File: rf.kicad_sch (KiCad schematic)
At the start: 59 parts, among them IC1 SX1255IWLTRT, J1 Antenna, U11 PE4312, U2 PE4312, U7 GRF5604, U9 SKY13330-397LF, Y1 32MHz

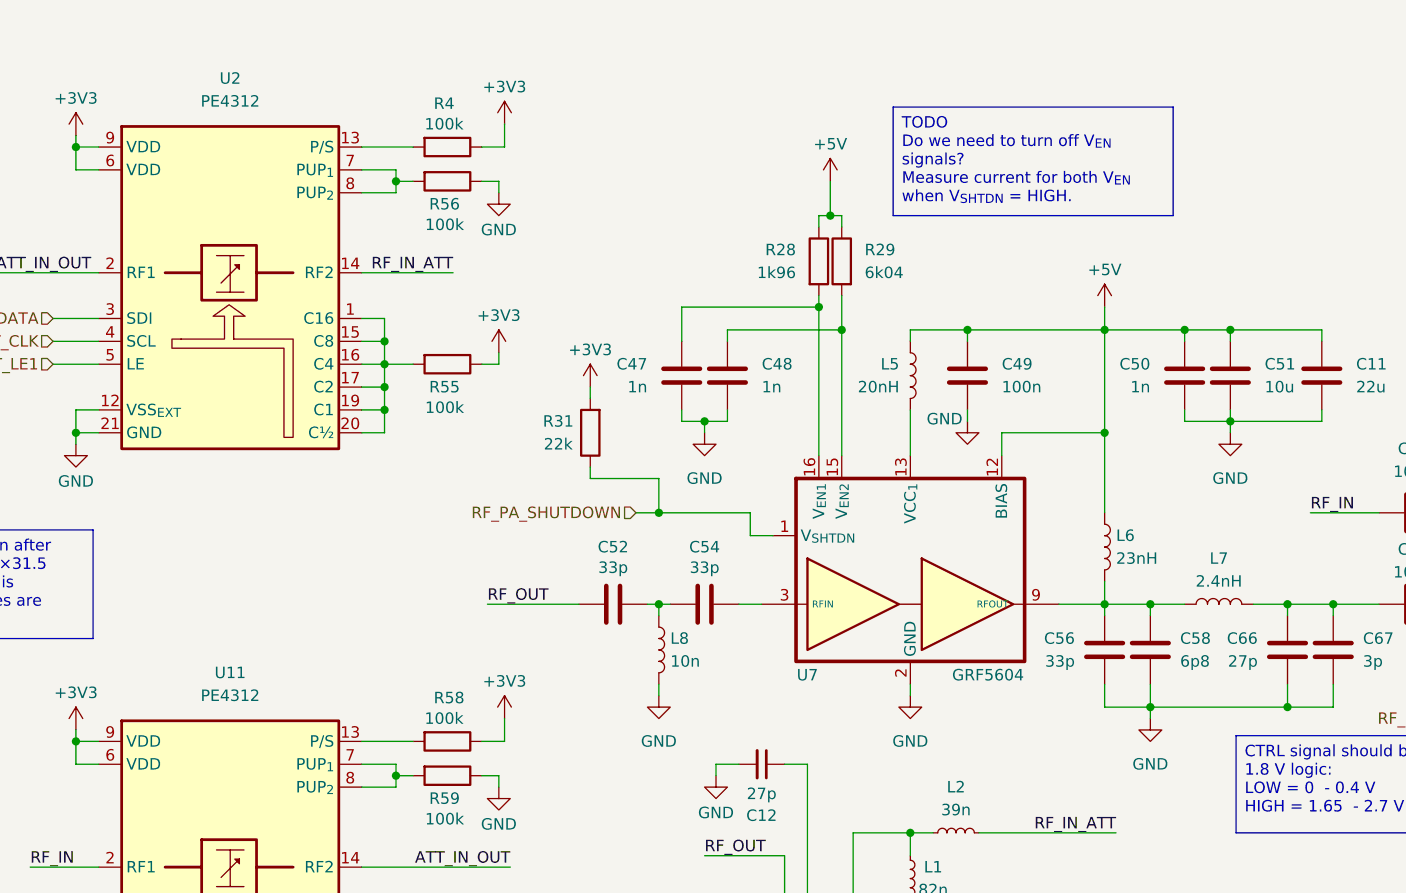
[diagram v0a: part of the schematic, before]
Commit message: Add `RF_PA_ENABLE` signal and MOSFETs to enable GRF5604
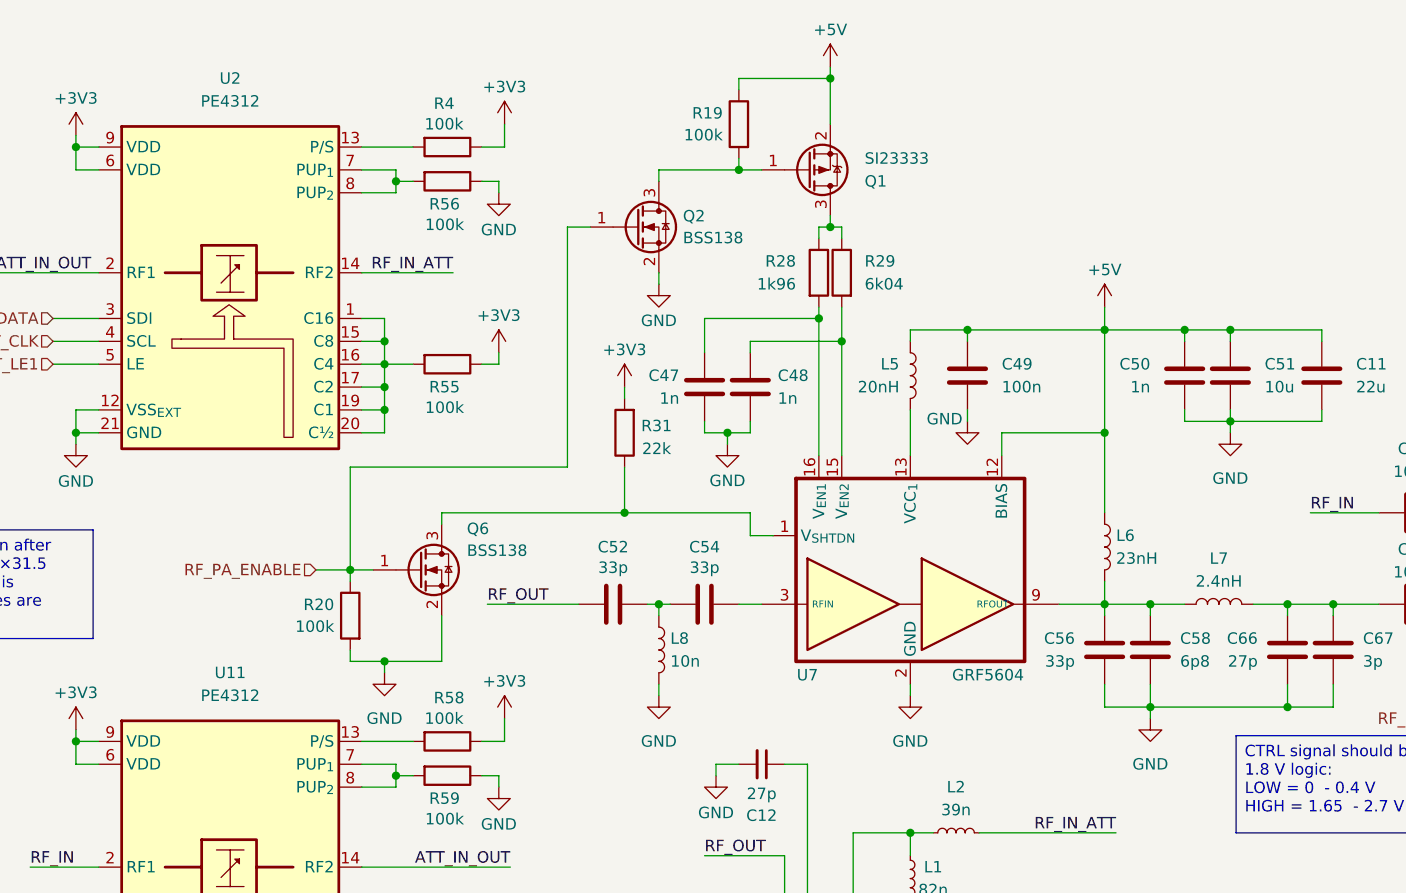
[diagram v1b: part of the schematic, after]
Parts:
- added Q1: SI23333, Package_TO_SOT_SMD:SOT-23, symbol Transistor_FET:Si2319CDS
- added Q2, Q6: BSS138, Package_TO_SOT_SMD:SOT-23, symbol Transistor_FET:BSS138
- added R19, R20: 100k, Resistor_SMD:R_0402_1005Metric, symbol Device:R
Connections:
- net +5V: now also Q1.2 (S), R19.1; no longer R28.1, R29.1
- net GND: now also Q2.2 (S), Q6.2 (S), R20.2
- net RF_PA_SHUTDOWN: no longer names the net of R31.1, U7.1 (V_{SHTDN})
- net RF_PA_SHUTDOWN: now also Q6.3 (D)
- new net: Q1.1 (G), Q2.3 (D), R19.2
- new net: Q1.3 (D), R28.1, R29.1
- new net RF_PA_ENABLE: Q2.1 (G), Q6.1 (G), R20.1
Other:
- moved on the sheet: C47, C48, R28, R29, R31

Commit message: Fix LCSC number of the GRF5604
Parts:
- U7: LCSC GRF5604 -> (none)
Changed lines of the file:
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@@
 		(on_board yes)
 		(dnp no)
-		(fields_autoplaced yes)
 		(property "Reference" "#PWR0146"
 			(at 82.55 91.44 0)
@@
 			)
 		)
-		(property "LCSC" "GRF5604"
+		(property "LCSC" ""
 			(at 147.32 77.47 0)
 			(effects

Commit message: Remove whitespaces in PN and MPN fields
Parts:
- C1, C2, C3, C4: PN 187-CL05B103KO5NNNC -> 187-CL05B103KO5NNNC
- C10, C13, C49, C5, C6, C7, C8, C9: PN 187-CL05B104KO5NNNC -> 187-CL05B104KO5NNNC
- C11: PN 187-CL31B226KPHNNNE -> 187-CL31B226KPHNNNE
- C12, C66: PN 603-CC402JRNPO9BN270 -> 603-CC402JRNPO9BN270
- C15, C47, C48, C50: PN 603-CC402JRNPO9BN102 -> 603-CC402JRNPO9BN102
- C51: PN 187-CL05A106MQ5NUNC -> 187-CL05A106MQ5NUNC
- IC1: PN 947-SX1255IWLTRT -> 947-SX1255IWLTRT
- Q2, Q6: PN 621-BSS138-7-F -> 621-BSS138-7-F
- U11, U2: PN 81-PE4312C-Z -> 81-PE4312C-Z
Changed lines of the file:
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@@
 			)
 		)
-		(property "PN" " 187-CL05B104KO5NNNC "
+		(property "PN" "187-CL05B104KO5NNNC"
 			(at 95.25 154.94 0)
 			(effects
@@
 			)
 		)
-		(property "PN" " 187-CL05B103KO5NNNC "
+		(property "PN" "187-CL05B103KO5NNNC"
 			(at 222.25 142.24 0)
 			(effects
@@
 			)
 		)
-		(property "PN" " 187-CL05B104KO5NNNC "
+		(property "PN" "187-CL05B104KO5NNNC"
 			(at 151.13 123.19 0)
 			(effects
@@
 			)
 		)
-		(property "PN" " 187-CL05A106MQ5NUNC "
+		(property "PN" "187-CL05A106MQ5NUNC"
 			(at 176.53 52.07 0)
 			(effects
@@
 			)
 		)
-		(property "PN" " 187-CL05B104KO5NNNC "
+		(property "PN" "187-CL05B104KO5NNNC"
 			(at 147.32 52.07 0)
 			(effects
@@
 			)
 		)
-		(property "PN" "81-PE4312C-Z "
+		(property "PN" "81-PE4312C-Z"
 			(at 50.8 92.71 0)
 			(effects
@@
 			)
 		)
-		(property "PN" " 187-CL05B104KO5NNNC "
+		(property "PN" "187-CL05B104KO5NNNC"
 			(at 271.78 142.24 0)
 			(effects
@@
 			)
 		)
-		(property "PN" " 187-CL05B104KO5NNNC "
+		(property "PN" "187-CL05B104KO5NNNC"
 			(at 77.47 154.94 0)
 			(effects
@@
 			)
 		)
-		(property "PN" " 187-CL05B104KO5NNNC "
+		(property "PN" "187-CL05B104KO5NNNC"
 			(at 260.35 142.24 0)
 			(effects
@@
 			)
 		)
-		(property "PN" " 603-CC402JRNPO9BN270 "
+		(property "PN" "603-CC402JRNPO9BN270"
 			(at 124.46 95.25 0)
 			(effects
@@
 			)
 		)
-		(property "PN" " 187-CL05B103KO5NNNC "
+		(property "PN" "187-CL05B103KO5NNNC"
 			(at 186.69 130.81 0)
 			(effects
@@
 			)
 		)
-		(property "PN" " 603-CC402JRNPO9BN102 "
+		(property "PN" "603-CC402JRNPO9BN102"
 			(at 171.45 52.07 0)
 			(effects
@@
 			)
 		)
-		(property "PN" " 603-CC402JRNPO9BN102 "
+		(property "PN" "603-CC402JRNPO9BN102"
 			(at 123.19 53.34 0)
 			(effects
@@
 			)
 		)
-		(property "PN" " 621-BSS138-7-F "
+		(property "PN" "621-BSS138-7-F"
 			(at 110.49 35.56 0)
 			(effects
@@
 			)
 		)
-		(property "PN" " 187-CL05B103KO5NNNC "
+		(property "PN" "187-CL05B103KO5NNNC"
 			(at 240.03 142.24 0)
 			(effects
@@
 			)
 		)
-		(property "PN" " 603-CC402JRNPO9BN102 "
+		(property "PN" "603-CC402JRNPO9BN102"
 			(at 118.11 53.34 0)
 			(effects
@@
 			)
 		)
-		(property "PN" " 621-BSS138-7-F "
+		(property "PN" "621-BSS138-7-F"
 			(at 86.36 73.66 0)
 			(effects
@@
 			)
 		)
-		(property "PN" " 187-CL31B226KPHNNNE "
+		(property "PN" "187-CL31B226KPHNNNE"
 			(at 186.69 52.07 0)
 			(effects
@@
 			)
 		)
-		(property "PN" " 187-CL05B104KO5NNNC "
+		(property "PN" "187-CL05B104KO5NNNC"
 			(at 248.92 142.24 0)
 			(effects
@@
 			)
 		)
-		(property "PN" "81-PE4312C-Z "
+		(property "PN" "81-PE4312C-Z"
 			(at 50.8 26.67 0)
 			(effects
@@
 			)
 		)
-		(property "PN" " 947-SX1255IWLTRT "
+		(property "PN" "947-SX1255IWLTRT"
 			(at 111.76 140.97 0)
 			(effects
@@
 			)
 		)
-		(property "PN" " 187-CL05B104KO5NNNC "
+		(property "PN" "187-CL05B104KO5NNNC"
 			(at 86.36 154.94 0)
 			(effects
@@
 			)
 		)
-		(property "PN" " 603-CC402JRNPO9BN270 "
+		(property "PN" "603-CC402JRNPO9BN270"
 			(at 182.88 82.55 0)
 			(effects
@@
 			)
 		)
-		(property "PN" " 187-CL05B103KO5NNNC "
+		(property "PN" "187-CL05B103KO5NNNC"
 			(at 231.14 142.24 0)
 			(effects
@@
 			)
 		)
-		(property "PN" " 603-CC402JRNPO9BN102 "
+		(property "PN" "603-CC402JRNPO9BN102"
 			(at 236.22 73.66 0)
 			(effects
